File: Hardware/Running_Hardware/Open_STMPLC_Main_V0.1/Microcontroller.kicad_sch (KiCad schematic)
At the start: 46 parts, among them J1 Conn_02x08_Odd_Even, J2 USB C, SW1 Switch, U1 STM32F407ZGTx, U3 TPS3430WDRC, U4 CH340C, Y1 48MHz, Y2 32.768kHz

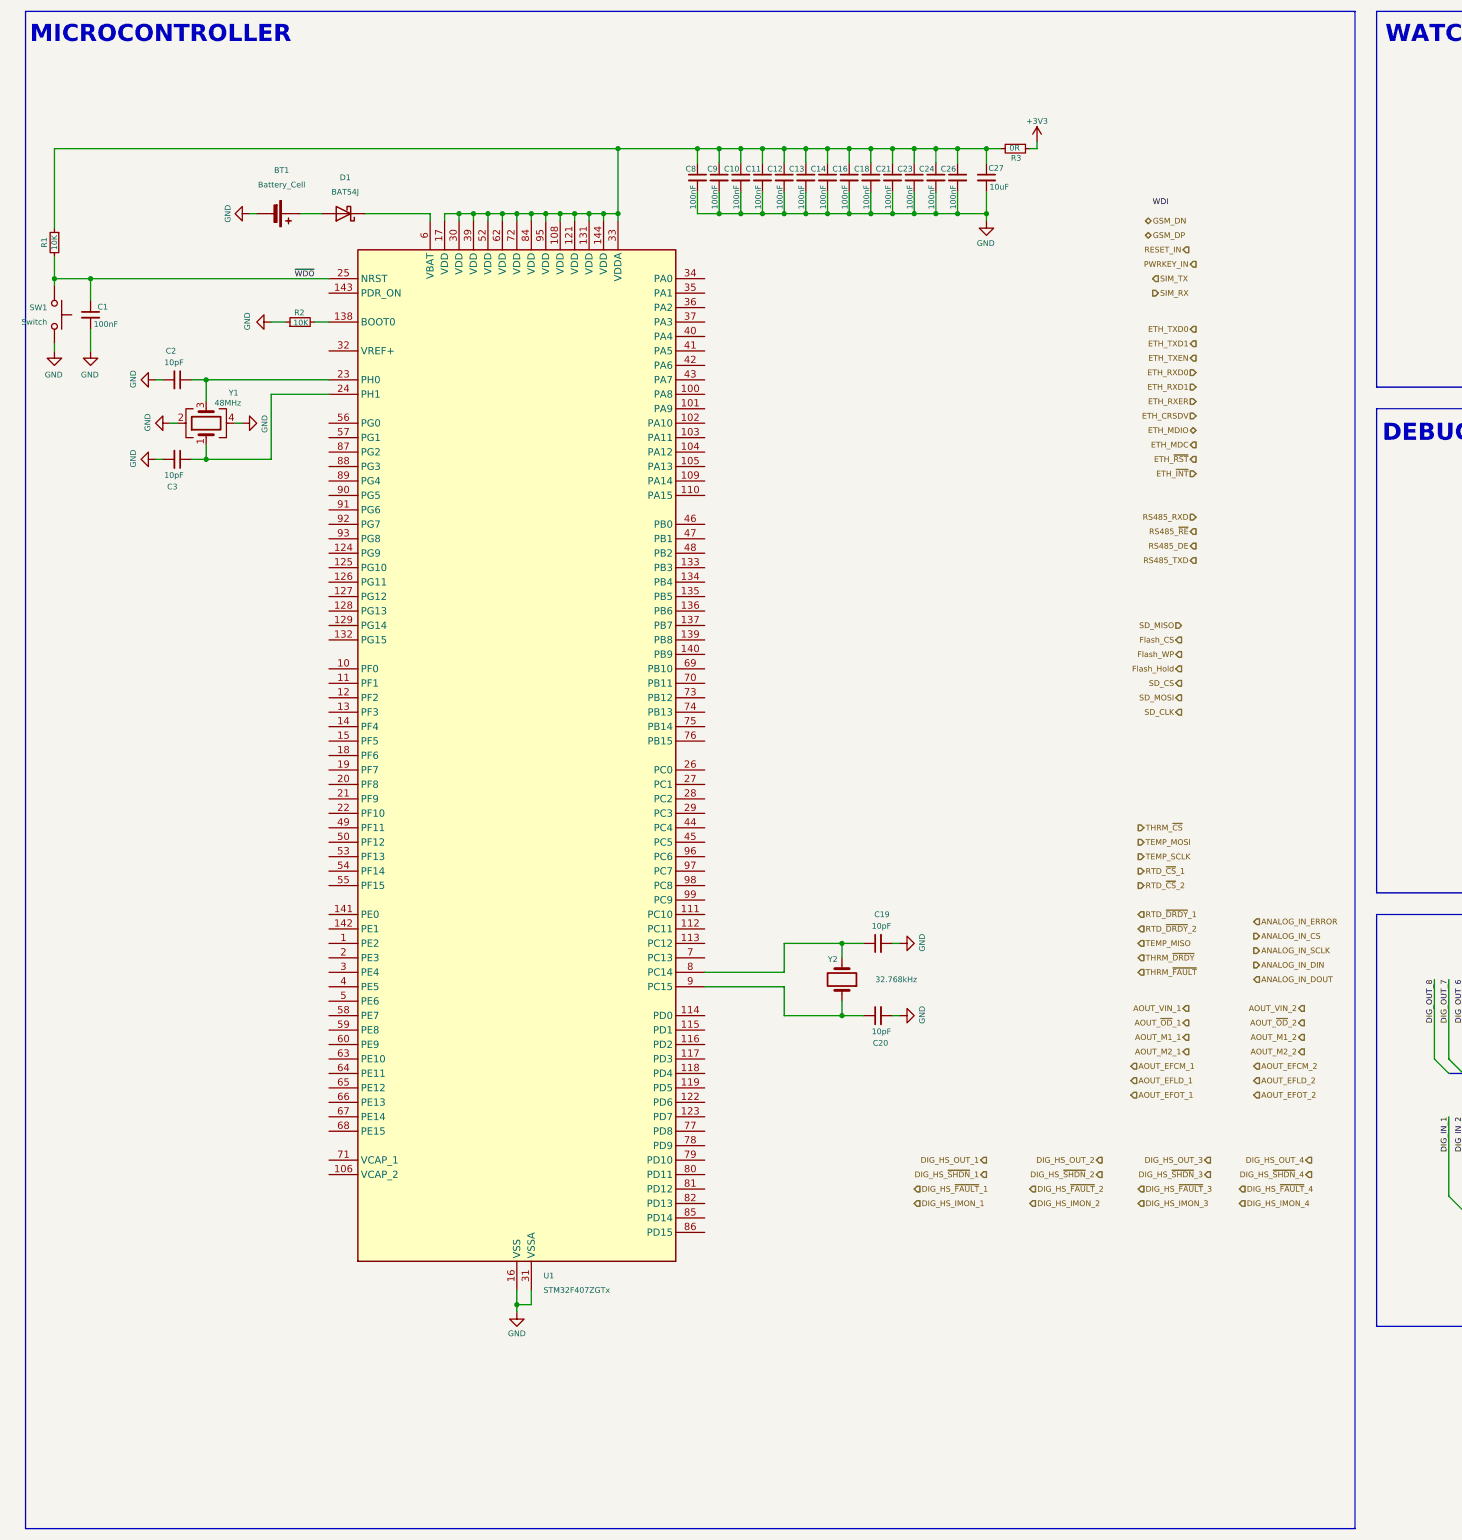
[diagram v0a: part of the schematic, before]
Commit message: Main PCB component placement
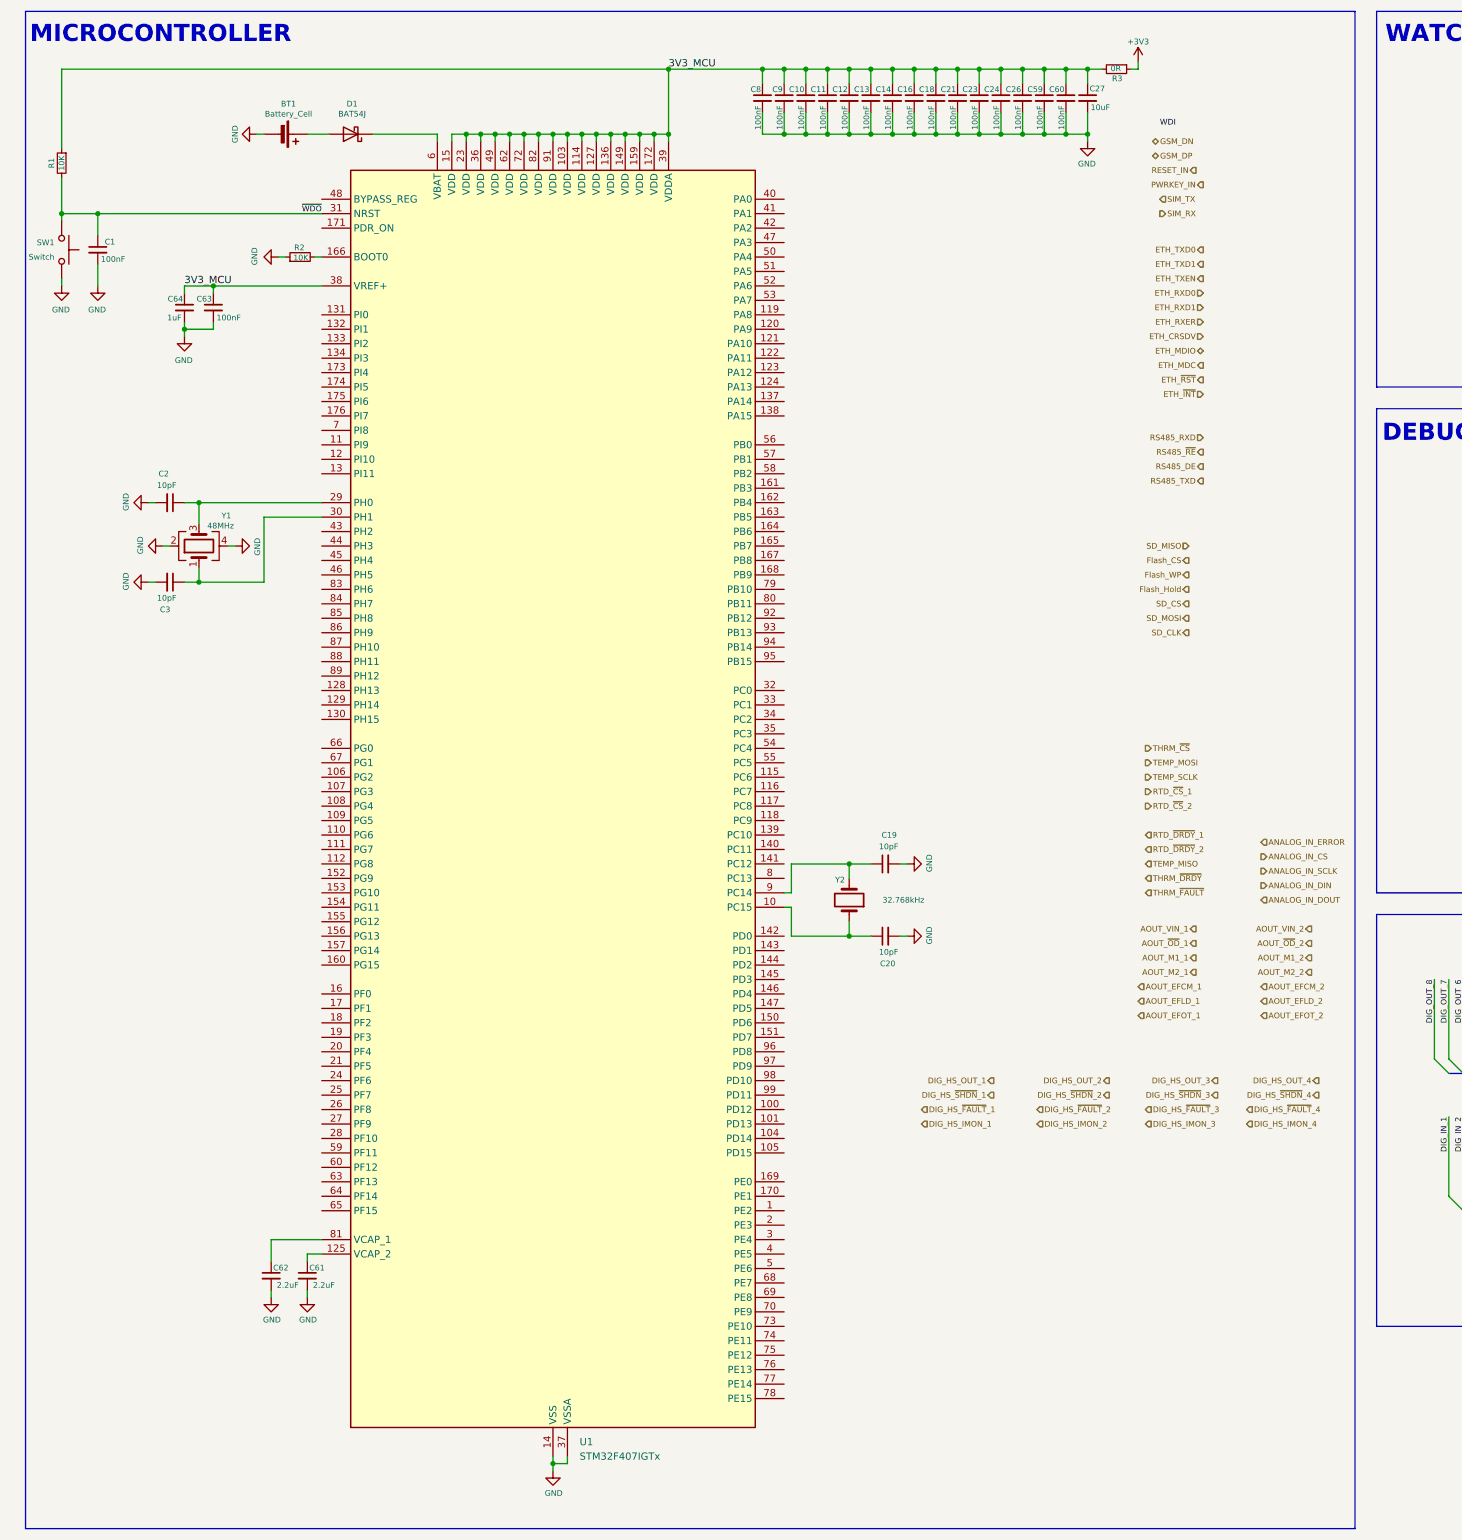
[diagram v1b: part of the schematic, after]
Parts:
- removed U1: STM32F407ZGTx, Package_QFP:LQFP-144_20x20mm_P0.5mm, symbol MCU_ST_STM32F4:STM32F407ZGTx
- added C59, C60, C63: 100nF, Capacitor_SMD:C_0603_1608Metric_Pad1.08x0.95mm_HandSolder, symbol Device:C_Small
- added C61, C62: 2.2uF, Capacitor_SMD:C_0603_1608Metric_Pad1.08x0.95mm_HandSolder, symbol Device:C_Small
- added C64: 1uF, Capacitor_SMD:C_0603_1608Metric_Pad1.08x0.95mm_HandSolder, symbol Device:C_Small
- added U1: STM32F407IGTx, Package_QFP:LQFP-176_24x24mm_P0.5mm, symbol MCU_ST_STM32F4:STM32F407IGTx
- SW1: footprint Button_Switch_SMD:SW_SPST_PTS810 -> Button_Switch_THT:SW_PUSH_6mm_H5mm
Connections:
- net GND: now also C59.2, C60.2, C61.2, C62.2, C63.2, C64.2, U1.102 (VSS), U1.113 (VSS), U1.126 (VSS), U1.135 (VSS), U1.14 (VSS), U1.148 (VSS), U1.158 (VSS), U1.22 (VSS), U1.37 (VSSA), U1.61 (VSS), U1.71 (VSS), U1.90 (VSS)
- net ~{WDO}: now also U1.31 (NRST)
- net at C3.1, Y1.1: now also U1.30 (PH1)
- net 3V3_MCU: now reaches C10.1, C11.1, C12.1, C13.1, C14.1, C16.1, C18.1, C21.1, C23.1, C24.1, C26.1, C27.1, C8.1, C9.1, R1.1, R3.2
- net 3V3_MCU: now also C59.1, C60.1, C63.1, C64.1, U1.103 (VDD), U1.114 (VDD), U1.127 (VDD), U1.136 (VDD), U1.149 (VDD), U1.15 (VDD), U1.159 (VDD), U1.172 (VDD), U1.23 (VDD), U1.36 (VDD), U1.38 (VREF+), U1.39 (VDDA), U1.49 (VDD), U1.62 (VDD), U1.72 (VDD), U1.82 (VDD), U1.91 (VDD)
- net at R2.2: now also U1.166 (BOOT0)
- net at C2.1, Y1.3: now also U1.29 (PH0)
- net at D1.1 (K): now also U1.6 (VBAT)
- net at C19.1, Y2.2: now also U1.9 (PC14)
- net at C20.1, Y2.1: now also U1.10 (PC15)
- new net: C61.1, U1.125 (VCAP_2)
- new net: C62.1, U1.81 (VCAP_1)
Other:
- moved on the sheet: BT1, C1, C10, C11, C12, C13, C14, C16, C18, C19, C2, C20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
